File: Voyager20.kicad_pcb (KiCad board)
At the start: 2 copper layers, 73 x 119.1 mm, 104 parts, among them Q1 Q_NPN_BEC, SW1 SW_Push, U1 ATmega32U2-AU, U2 PRTR5V0U2X, Y1 16MHz

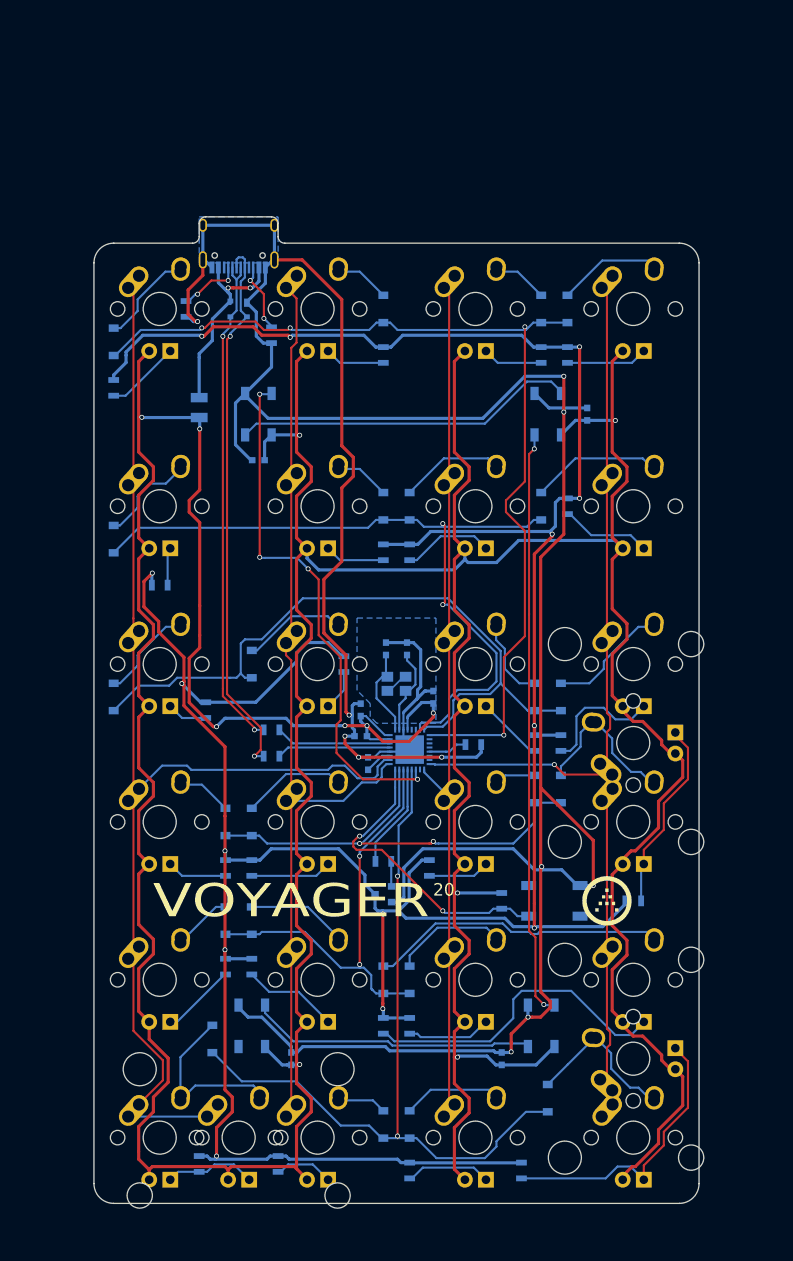
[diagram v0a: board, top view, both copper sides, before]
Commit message: Route 3700 variant
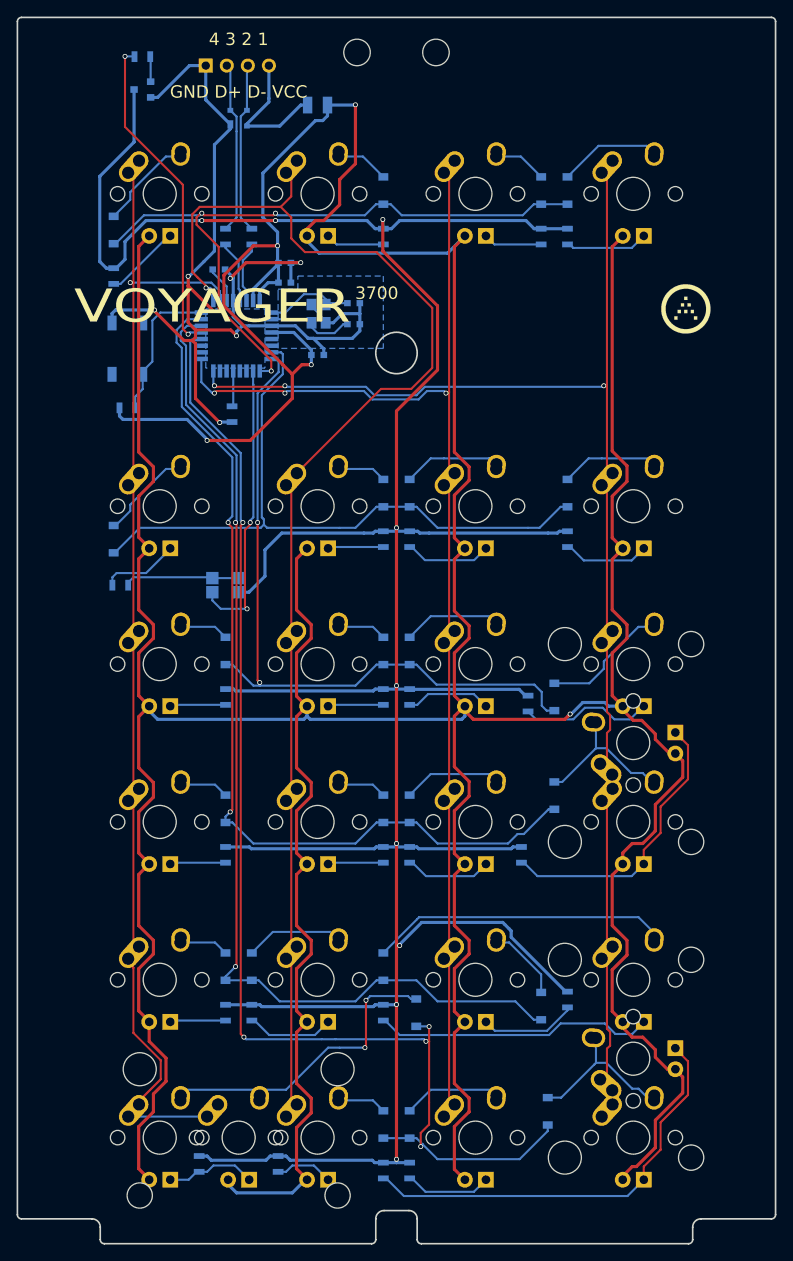
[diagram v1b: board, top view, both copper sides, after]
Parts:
- removed CR1, CR2, CR3, CR4: 0.1u, Capacitors_SMD:C_0603
- removed D18, D23, D24, D9: WS2812B, LEDs:LED_WS2812B-PLCC4
- removed R4, R6: 5.1k, Resistors_SMD:R_0805
- removed USB1: HRO-TYPE-C-31-M-12, Type-C:HRO-TYPE-C-31-M-12-Assembly
- added J1: Conn_01x04, Pin_Headers:Pin_Header_Straight_1x04_Pitch2.54mm, B.Cu at (53.2, -13.5)
- added JP1: JP-INDICATOR, random-keyboard-parts:Jumper-UserFriendly-Small, B.Cu at (54.0, 49.2)
- added JP2: JP-BLIGHT, random-keyboard-parts:Jumper-UserFriendly-Small, B.Cu at (57.1, 49.2)
- added REF**: outline, locallib:outline, F.Cu at (30.4, -19.3)
- added REF**: MountingHole_3.2mm_M3, Mounting_Holes:MountingHole_3.2mm_M3, F.Cu at (71.4, -15.1)
- added REF**: MountingHole_3.2mm_M3, Mounting_Holes:MountingHole_3.2mm_M3, F.Cu at (81.0, -15.1)
- U1: footprint Housings_DFN_QFN:QFN-32-1EP_5x5mm_Pitch0.5mm -> Housings_QFP:TQFP-32_7x7mm_Pitch0.8mm
- moved Q1 101.4 mm to (45.5, -10.6)
- moved R27 101.4 mm to (45.5, -14.6)
- moved SW1 84.2 mm to (43.7, 20.7), turned to 90 degrees
- moved R1 74.7 mm to (43.7, 27.8), turned to 0 degrees
- moved G*** 72.1 mm to (111.1, 15.9)
- moved R3 63.0 mm to (55.6, 7.14), turned to 270 degrees
- moved C3 62.3 mm to (54.8, 11.1), turned to 0 degrees
- moved R2 59.6 mm to (58.7, 7.14), turned to 90 degrees
- moved C5 55.5 mm to (62.7, 12.7), turned to 0 degrees
- moved C6 54.7 mm to (62.7, 10.3), turned to 0 degrees
- moved U1 54.1 mm to (56.9, 19.1), turned to 180 degrees
- moved R5 49.4 mm to (56.4, 28.6), turned to 90 degrees
- moved Y1 45.7 mm to (66.8, 16.4), turned to 270 degrees
- moved C4 43.6 mm to (66.7, 21.4), turned to 0 degrees
- moved C1 41.9 mm to (71.0, 15.2), turned to 0 degrees
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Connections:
- net Net-(MX1-Pad4) renamed NLOCKLED
- R7 pad 2: LEDGND -> Net-(JP1-Pad1)
- U1 pad 10: Net-(U1-Pad10) -> NLCKLED
- U1 pad 19: RGBLED -> Net-(U1-Pad19)
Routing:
- net GND: track 396.1 -> 131.7 mm, vias 11 -> 6
- net ROW3: track 52.5 -> 126.6 mm
- net Net-(D18-Pad2): track 71.1 -> 0.00 mm, vias 2 -> 0
- net RGBLED: track 64.0 -> 0.00 mm, vias 4 -> 0
- net ROW4: track 93.6 -> 150.7 mm, vias 2 -> 5
- net ROW2: track 55.6 -> 111.1 mm
- net Net-(J1-Pad2): track 66.7 -> 20.7 mm, vias 2 -> 0
- net COL3: track 124.4 -> 166.2 mm, vias 1 -> 3
- net COL2: track 107.4 -> 149.0 mm, vias 0 -> 3
- net Net-(D18-Pad4): track 41.5 -> 0.00 mm
- net Net-(J1-Pad3): track 61.0 -> 20.6 mm, vias 2 -> 0
- net COL1: track 118.1 -> 158.1 mm, vias 0 -> 1
- net ROWFN: track 119.8 -> 82.8 mm, vias 4 -> 3
- net NLCKLED: track 0.00 -> 34.8 mm, vias 0 -> 2
- net Net-(D23-Pad2): track 34.6 -> 0.00 mm
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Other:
- board size 73 x 119.1 mm -> 91.5 x 148 mm
- board text added: "1 2 3 4"
- board text added: "3700"
- board text added: "4 3 2 1"
- board text added: "BACKL"
- board text added: "Connection Options a) Hardwire USB cable to USB pads. Optionally zip-tie the cable to the pcb using the hole provided for strength. b) Mount a Mini-XLR connector on the PS2 passthrough hole. Wire to the USB pads, following the numbered order."
- board text added: "GND D+ D- VCC"
- board text added: "IND"
- board text added: "VCC D- D+ GND"
- board text removed: "20"
- board text removed: "Voyager20 PCB Rev 1.0 20190126 kb.ai03.me"
